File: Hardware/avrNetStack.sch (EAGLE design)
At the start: 34 parts, among them IC1 MEGA32-P, IC2 ENC28J60SP, Q1 16M, Q2 25M

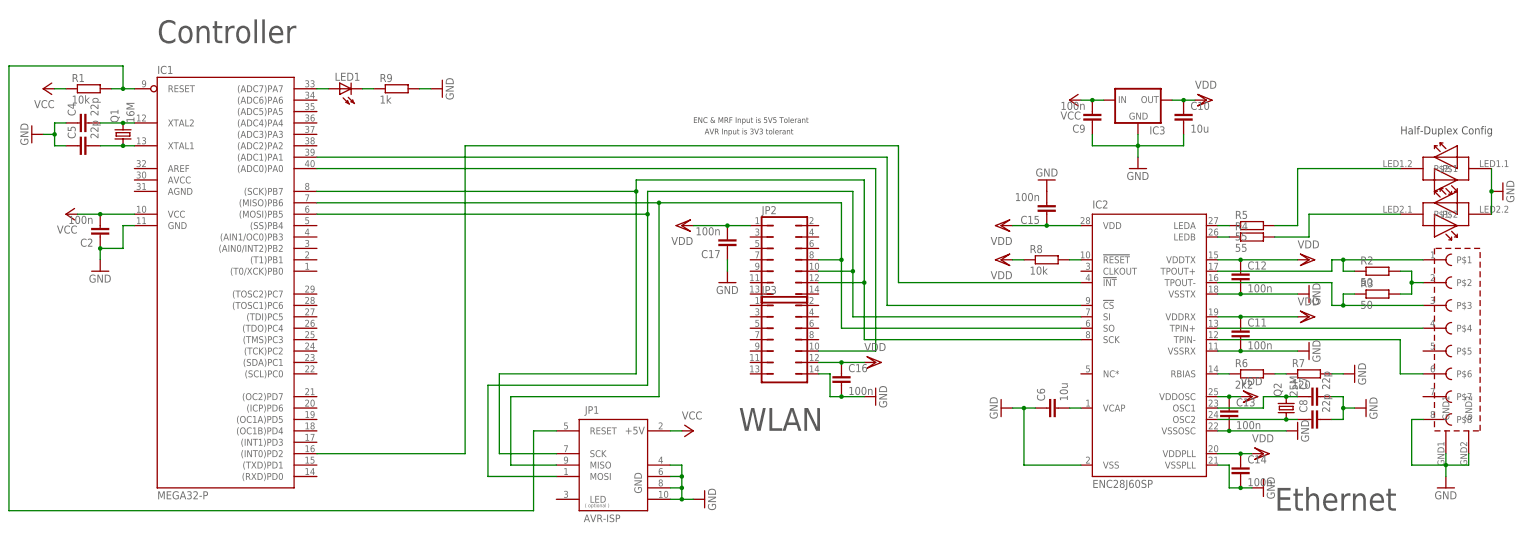
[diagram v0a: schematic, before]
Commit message: Built Test Hardware.
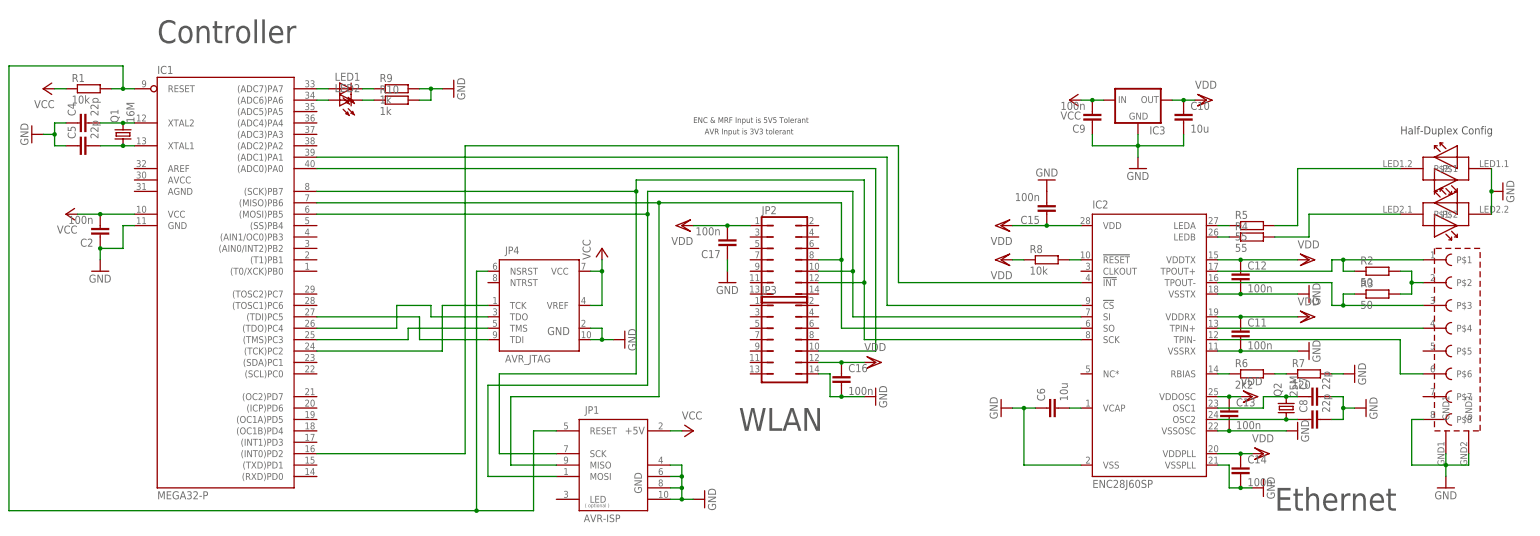
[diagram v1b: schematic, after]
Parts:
- added JP4: AVR_JTAG, 0_RN:AVR_JTAG
- added LED2: (no value), led:LED5MM
- added R10: 1k, resistor:R-EU_0204/7
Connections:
- new net N$28: LED2.C, R10.1
- new net N$29: IC1.(TDI)PC5, JP4.TDI
- new net N$30: IC1.(TMS)PC3, JP4.TMS
- new net N$31: IC1.(TDO)PC4, JP4.TDO
- new net N$32: IC1.(TCK)PC2, JP4.TCK
- new net N$9: IC1.(ADC6)PA6, LED2.A
- net GND: now also JP4.GND, JP4.GND@1, R10.2
- net N$1: now also JP4.NSRST
- net VCC: now also JP4.VCC, JP4.VREF
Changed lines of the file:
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@@
 <part name="P+4" library="supply1" deviceset="VCC" device=""/>
 <part name="GND17" library="supply1" deviceset="GND" device=""/>
+<part name="LED2" library="led" deviceset="LED" device="5MM"/>
+<part name="R10" library="resistor" deviceset="R-EU_" device="0204/7" value="1k"/>
+<part name="JP4" library="0_RN" deviceset="AVR_JTAG" device=""/>
+<part name="P+5" library="supply1" deviceset="VCC" device=""/>
+<part name="GND18" library="supply1" deviceset="GND" device=""/>
 </parts>
 <sheets>
@@
 <instance part="LED1" gate="G$1" x="96.52" y="119.38" rot="R90"/>
 <instance part="R9" gate="G$1" x="109.22" y="119.38"/>
-<instance part="GND13" gate="1" x="119.38" y="119.38" rot="R90"/>
+<instance part="GND13" gate="1" x="121.92" y="119.38" rot="R90"/>
 <instance part="IC3" gate="1" x="274.32" y="116.84"/>
 <instance part="C9" gate="G$1" x="264.16" y="111.76" rot="R180"/>
@@
 <instance part="P+4" gate="VCC" x="35.56" y="91.44" rot="R90"/>
 <instance part="GND17" gate="1" x="27.94" y="109.22" rot="R270"/>
+<instance part="LED2" gate="G$1" x="96.52" y="116.84" rot="R90"/>
+<instance part="R10" gate="G$1" x="109.22" y="116.84"/>
+<instance part="JP4" gate="JP" x="142.24" y="71.12"/>
+<instance part="P+5" gate="VCC" x="154.94" y="83.82"/>
+<instance part="GND18" gate="1" x="160.02" y="63.5" rot="R90"/>
 </instances>
 <busses>
@@
 <wire x1="144.78" y1="43.18" x2="139.7" y2="43.18" width="0.1524" layer="91"/>
 <wire x1="139.7" y1="43.18" x2="139.7" y2="25.4" width="0.1524" layer="91"/>
-<wire x1="139.7" y1="25.4" x2="22.86" y2="25.4" width="0.1524" layer="91"/>
+<wire x1="139.7" y1="25.4" x2="127" y2="25.4" width="0.1524" layer="91"/>
+<wire x1="127" y1="25.4" x2="22.86" y2="25.4" width="0.1524" layer="91"/>
 <wire x1="22.86" y1="25.4" x2="22.86" y2="124.46" width="0.1524" layer="91"/>
 <pinref part="IC1" gate="G$1" pin="RESET"/>
@@
 <wire x1="48.26" y1="124.46" x2="48.26" y2="119.38" width="0.1524" layer="91"/>
 <junction x="48.26" y="119.38"/>
+<pinref part="JP4" gate="JP" pin="NSRST"/>
+<wire x1="129.54" y1="78.74" x2="127" y2="78.74" width="0.1524" layer="91"/>
+<wire x1="127" y1="78.74" x2="127" y2="25.4" width="0.1524" layer="91"/>
+<junction x="127" y="25.4"/>
 </segment>
 </net>
@@
 <pinref part="P+1" gate="VCC" pin="VCC"/>
 <wire x1="35.56" y1="119.38" x2="33.02" y2="119.38" width="0.1524" layer="91"/>
+</segment>
+<segment>
+<pinref part="JP4" gate="JP" pin="VREF"/>
+<wire x1="152.4" y1="71.12" x2="154.94" y2="71.12" width="0.1524" layer="91"/>
+<wire x1="154.94" y1="71.12" x2="154.94" y2="78.74" width="0.1524" layer="91"/>
+<pinref part="JP4" gate="JP" pin="VCC"/>
+<wire x1="154.94" y1="78.74" x2="152.4" y2="78.74" width="0.1524" layer="91"/>
+<pinref part="P+5" gate="VCC" pin="VCC"/>
+<wire x1="154.94" y1="78.74" x2="154.94" y2="81.28" width="0.1524" layer="91"/>
+<junction x="154.94" y="78.74"/>
 </segment>
 </net>
@@
 <pinref part="GND13" gate="1" pin="GND"/>
 <wire x1="114.3" y1="119.38" x2="116.84" y2="119.38" width="0.1524" layer="91"/>
+<pinref part="R10" gate="G$1" pin="2"/>
+<wire x1="116.84" y1="119.38" x2="119.38" y2="119.38" width="0.1524" layer="91"/>
+<wire x1="114.3" y1="116.84" x2="116.84" y2="116.84" width="0.1524" layer="91"/>
+<wire x1="116.84" y1="116.84" x2="116.84" y2="119.38" width="0.1524" layer="91"/>
+<junction x="116.84" y="119.38"/>
 </segment>
 <segment>
@@
 <wire x1="33.02" y1="106.68" x2="33.02" y2="109.22" width="0.1524" layer="91"/>
 <junction x="33.02" y="109.22"/>
+</segment>
+<segment>
+<pinref part="GND18" gate="1" pin="GND"/>
+<wire x1="157.48" y1="63.5" x2="154.94" y2="63.5" width="0.1524" layer="91"/>
+<wire x1="154.94" y1="63.5" x2="154.94" y2="66.04" width="0.1524" layer="91"/>
+<pinref part="JP4" gate="JP" pin="GND"/>
+<wire x1="154.94" y1="66.04" x2="152.4" y2="66.04" width="0.1524" layer="91"/>
+<pinref part="JP4" gate="JP" pin="GND@1"/>
+<wire x1="152.4" y1="63.5" x2="154.94" y2="63.5" width="0.1524" layer="91"/>
+<junction x="154.94" y="63.5"/>
 </segment>
 </net>
@@
 </segment>
 </net>
+<net name="N$9" class="0">
+<segment>
+<pinref part="IC1" gate="G$1" pin="(ADC6)PA6"/>
+<pinref part="LED2" gate="G$1" pin="A"/>
+<wire x1="91.44" y1="116.84" x2="93.98" y2="116.84" width="0.1524" layer="91"/>
+</segment>
+</net>
+<net name="N$28" class="0">
+<segment>
+<pinref part="LED2" gate="G$1" pin="C"/>
+<pinref part="R10" gate="G$1" pin="1"/>
+<wire x1="101.6" y1="116.84" x2="104.14" y2="116.84" width="0.1524" layer="91"/>
+</segment>
+</net>
+<net name="N$29" class="0">
+<segment>
+<pinref part="IC1" gate="G$1" pin="(TDI)PC5"/>
+<wire x1="91.44" y1="68.58" x2="114.3" y2="68.58" width="0.1524" layer="91"/>
+<wire x1="114.3" y1="68.58" x2="114.3" y2="63.5" width="0.1524" layer="91"/>
+<pinref part="JP4" gate="JP" pin="TDI"/>
+<wire x1="114.3" y1="63.5" x2="129.54" y2="63.5" width="0.1524" layer="91"/>
+</segment>
+</net>
+<net name="N$30" class="0">
+<segment>
+<pinref part="JP4" gate="JP" pin="TMS"/>
+<wire x1="129.54" y1="66.04" x2="111.76" y2="66.04" width="0.1524" layer="91"/>
+<wire x1="111.76" y1="66.04" x2="111.76" y2="63.5" width="0.1524" layer="91"/>
+<pinref part="IC1" gate="G$1" pin="(TMS)PC3"/>
+<wire x1="111.76" y1="63.5" x2="91.44" y2="63.5" width="0.1524" layer="91"/>
+</segment>
+</net>
+<net name="N$31" class="0">
+<segment>
+<pinref part="IC1" gate="G$1" pin="(TDO)PC4"/>
+<wire x1="91.44" y1="66.04" x2="109.22" y2="66.04" width="0.1524" layer="91"/>
+<wire x1="109.22" y1="66.04" x2="109.22" y2="71.12" width="0.1524" layer="91"/>
+<wire x1="109.22" y1="71.12" x2="116.84" y2="71.12" width="0.1524" layer="91"/>
+<wire x1="116.84" y1="71.12" x2="116.84" y2="68.58" width="0.1524" layer="91"/>
+<pinref part="JP4" gate="JP" pin="TDO"/>
+<wire x1="116.84" y1="68.58" x2="129.54" y2="68.58" width="0.1524" layer="91"/>
+</segment>
+</net>
+<net name="N$32" class="0">
+<segment>
+<pinref part="JP4" gate="JP" pin="TCK"/>
+<wire x1="129.54" y1="71.12" x2="119.38" y2="71.12" width="0.1524" layer="91"/>
+<wire x1="119.38" y1="71.12" x2="119.38" y2="60.96" width="0.1524" layer="91"/>
+<pinref part="IC1" gate="G$1" pin="(TCK)PC2"/>
+<wire x1="119.38" y1="60.96" x2="91.44" y2="60.96" width="0.1524" layer="91"/>
+</segment>
+</net>

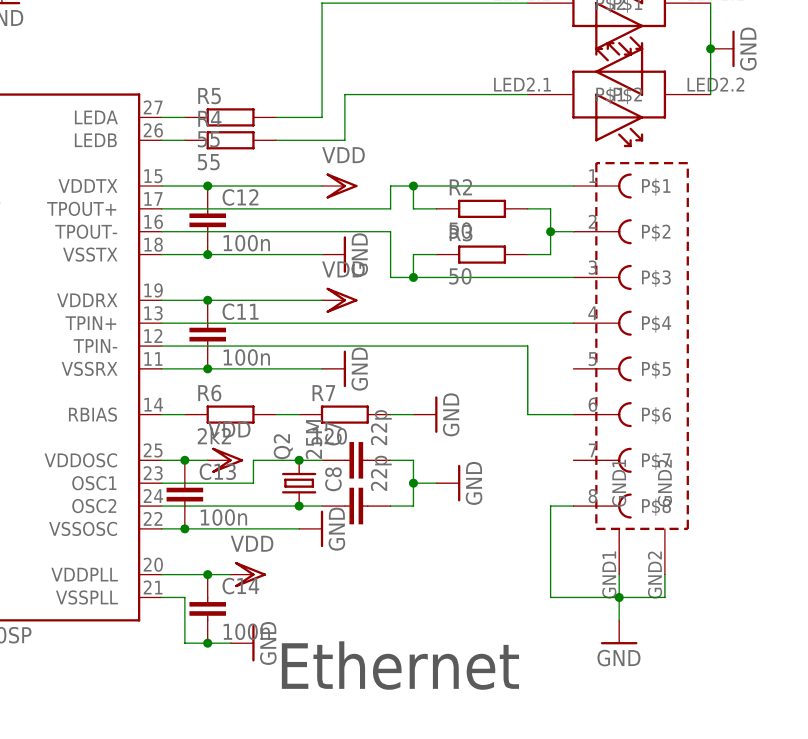
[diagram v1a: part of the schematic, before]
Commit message: Extended capabilities.
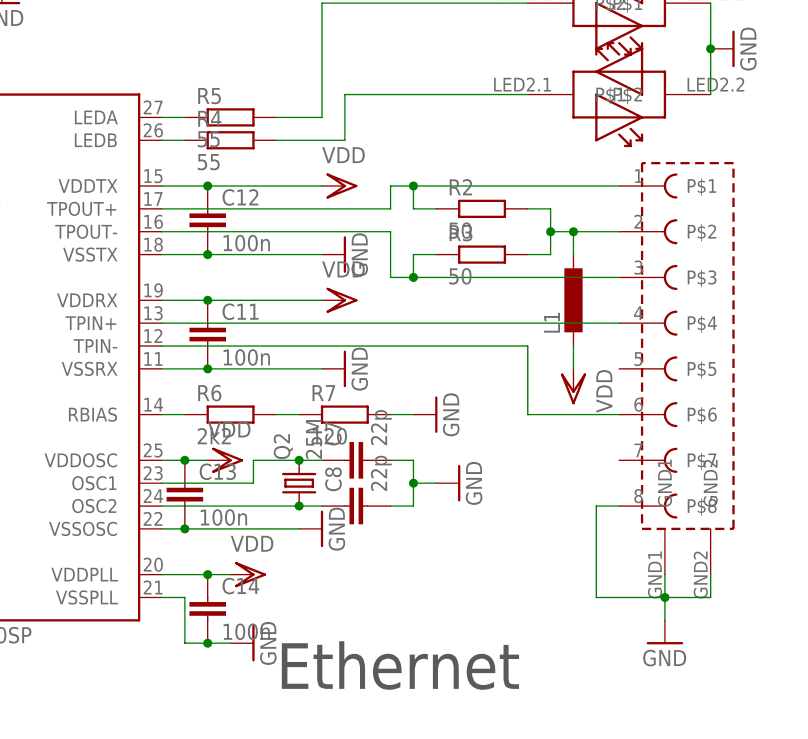
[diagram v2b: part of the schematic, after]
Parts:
- added L1: (no value), resistor:L-EU0204/7
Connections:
- net N$16: now also L1.1
- net VDD: now also L1.2
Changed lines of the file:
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@@
 <part name="P+5" library="supply1" deviceset="VCC" device=""/>
 <part name="GND18" library="supply1" deviceset="GND" device=""/>
+<part name="L1" library="resistor" deviceset="L-EU" device="0204/7"/>
+<part name="VDD10" library="supply1" deviceset="VDD" device=""/>
 </parts>
 <sheets>
@@
 <instance part="R2" gate="G$1" x="327.66" y="78.74"/>
 <instance part="R3" gate="G$1" x="327.66" y="73.66"/>
-<instance part="U$1" gate="G$1" x="345.44" y="66.04"/>
+<instance part="U$1" gate="G$1" x="350.52" y="66.04"/>
 <instance part="U$1" gate="G$2" x="342.9" y="104.14" rot="R180"/>
 <instance part="U$1" gate="G$3" x="342.9" y="88.9"/>
-<instance part="GND5" gate="1" x="342.9" y="30.48"/>
+<instance part="GND5" gate="1" x="347.98" y="30.48"/>
 <instance part="R4" gate="G$1" x="299.72" y="86.36"/>
 <instance part="R5" gate="G$1" x="299.72" y="88.9"/>
@@
 <instance part="P+5" gate="VCC" x="154.94" y="83.82"/>
 <instance part="GND18" gate="1" x="160.02" y="63.5" rot="R90"/>
+<instance part="L1" gate="G$1" x="337.82" y="68.58"/>
+<instance part="VDD10" gate="G$1" x="337.82" y="58.42" rot="R180"/>
 </instances>
 <busses>
@@
 <pinref part="GND5" gate="1" pin="GND"/>
 <pinref part="U$1" gate="G$1" pin="GND1"/>
-<wire x1="342.9" y1="33.02" x2="342.9" y2="35.56" width="0.1524" layer="91"/>
+<wire x1="347.98" y1="33.02" x2="347.98" y2="35.56" width="0.1524" layer="91"/>
 <pinref part="U$1" gate="G$1" pin="GND2"/>
-<wire x1="342.9" y1="35.56" x2="342.9" y2="38.1" width="0.1524" layer="91"/>
-<wire x1="342.9" y1="35.56" x2="347.98" y2="35.56" width="0.1524" layer="91"/>
 <wire x1="347.98" y1="35.56" x2="347.98" y2="38.1" width="0.1524" layer="91"/>
-<junction x="342.9" y="35.56"/>
+<wire x1="347.98" y1="35.56" x2="353.06" y2="35.56" width="0.1524" layer="91"/>
+<wire x1="353.06" y1="35.56" x2="353.06" y2="38.1" width="0.1524" layer="91"/>
+<junction x="347.98" y="35.56"/>
 <pinref part="U$1" gate="G$1" pin="P$8"/>
-<wire x1="337.82" y1="45.72" x2="335.28" y2="45.72" width="0.1524" layer="91"/>
-<wire x1="335.28" y1="45.72" x2="335.28" y2="35.56" width="0.1524" layer="91"/>
-<wire x1="335.28" y1="35.56" x2="342.9" y2="35.56" width="0.1524" layer="91"/>
+<wire x1="342.9" y1="45.72" x2="340.36" y2="45.72" width="0.1524" layer="91"/>
+<wire x1="340.36" y1="45.72" x2="340.36" y2="35.56" width="0.1524" layer="91"/>
+<wire x1="340.36" y1="35.56" x2="347.98" y2="35.56" width="0.1524" layer="91"/>
 </segment>
 <segment>
@@
 <wire x1="317.5" y1="81.28" x2="320.04" y2="81.28" width="0.1524" layer="91"/>
 <pinref part="R2" gate="G$1" pin="1"/>
-<wire x1="320.04" y1="81.28" x2="337.82" y2="81.28" width="0.1524" layer="91"/>
+<wire x1="320.04" y1="81.28" x2="342.9" y2="81.28" width="0.1524" layer="91"/>
 <wire x1="322.58" y1="78.74" x2="320.04" y2="78.74" width="0.1524" layer="91"/>
 <wire x1="320.04" y1="78.74" x2="320.04" y2="81.28" width="0.1524" layer="91"/>
@@
 <net name="N$10" class="0">
 <segment>
-<wire x1="337.82" y1="71.12" x2="320.04" y2="71.12" width="0.1524" layer="91"/>
+<wire x1="342.9" y1="71.12" x2="320.04" y2="71.12" width="0.1524" layer="91"/>
 <wire x1="320.04" y1="71.12" x2="317.5" y2="71.12" width="0.1524" layer="91"/>
 <wire x1="317.5" y1="71.12" x2="317.5" y2="76.2" width="0.1524" layer="91"/>
@@
 <segment>
 <pinref part="IC2" gate="G$1" pin="TPIN+"/>
-<wire x1="292.1" y1="66.04" x2="337.82" y2="66.04" width="0.1524" layer="91"/>
+<wire x1="292.1" y1="66.04" x2="342.9" y2="66.04" width="0.1524" layer="91"/>
 <pinref part="U$1" gate="G$1" pin="P$4"/>
 </segment>
@@
 <wire x1="335.28" y1="76.2" x2="337.82" y2="76.2" width="0.1524" layer="91"/>
 <pinref part="R3" gate="G$1" pin="2"/>
+<wire x1="337.82" y1="76.2" x2="342.9" y2="76.2" width="0.1524" layer="91"/>
 <wire x1="332.74" y1="73.66" x2="335.28" y2="73.66" width="0.1524" layer="91"/>
 <wire x1="335.28" y1="73.66" x2="335.28" y2="76.2" width="0.1524" layer="91"/>
 <junction x="335.28" y="76.2"/>
 <pinref part="U$1" gate="G$1" pin="P$2"/>
+<pinref part="L1" gate="G$1" pin="1"/>
+<wire x1="337.82" y1="73.66" x2="337.82" y2="76.2" width="0.1524" layer="91"/>
+<junction x="337.82" y="76.2"/>
 </segment>
 </net>
 <net name="N$17" class="0">
 <segment>
-<wire x1="337.82" y1="55.88" x2="332.74" y2="55.88" width="0.1524" layer="91"/>
+<wire x1="342.9" y1="55.88" x2="332.74" y2="55.88" width="0.1524" layer="91"/>
 <wire x1="332.74" y1="55.88" x2="332.74" y2="63.5" width="0.1524" layer="91"/>
 <pinref part="IC2" gate="G$1" pin="TPIN-"/>
@@
 <junction x="208.28" y="58.42"/>
 </segment>
-</net>
+<segment>
+<pinref part="VDD10" gate="G$1" pin="VDD"/>
+<pinref part="L1" gate="G$1" pin="2"/>
+<wire x1="337.82" y1="60.96" x2="337.82" y2="63.5" width="0.1524" layer="91"/>
+</segment>
+</net>
